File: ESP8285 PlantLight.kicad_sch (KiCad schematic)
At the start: 43 parts, among them J1 Screw_Terminal_01x01, J2 Screw_Terminal_01x01, Q1 P-Chan Mosfet, U1 ESP8285, U2 RT9193-33GB, Y1 26Mhz

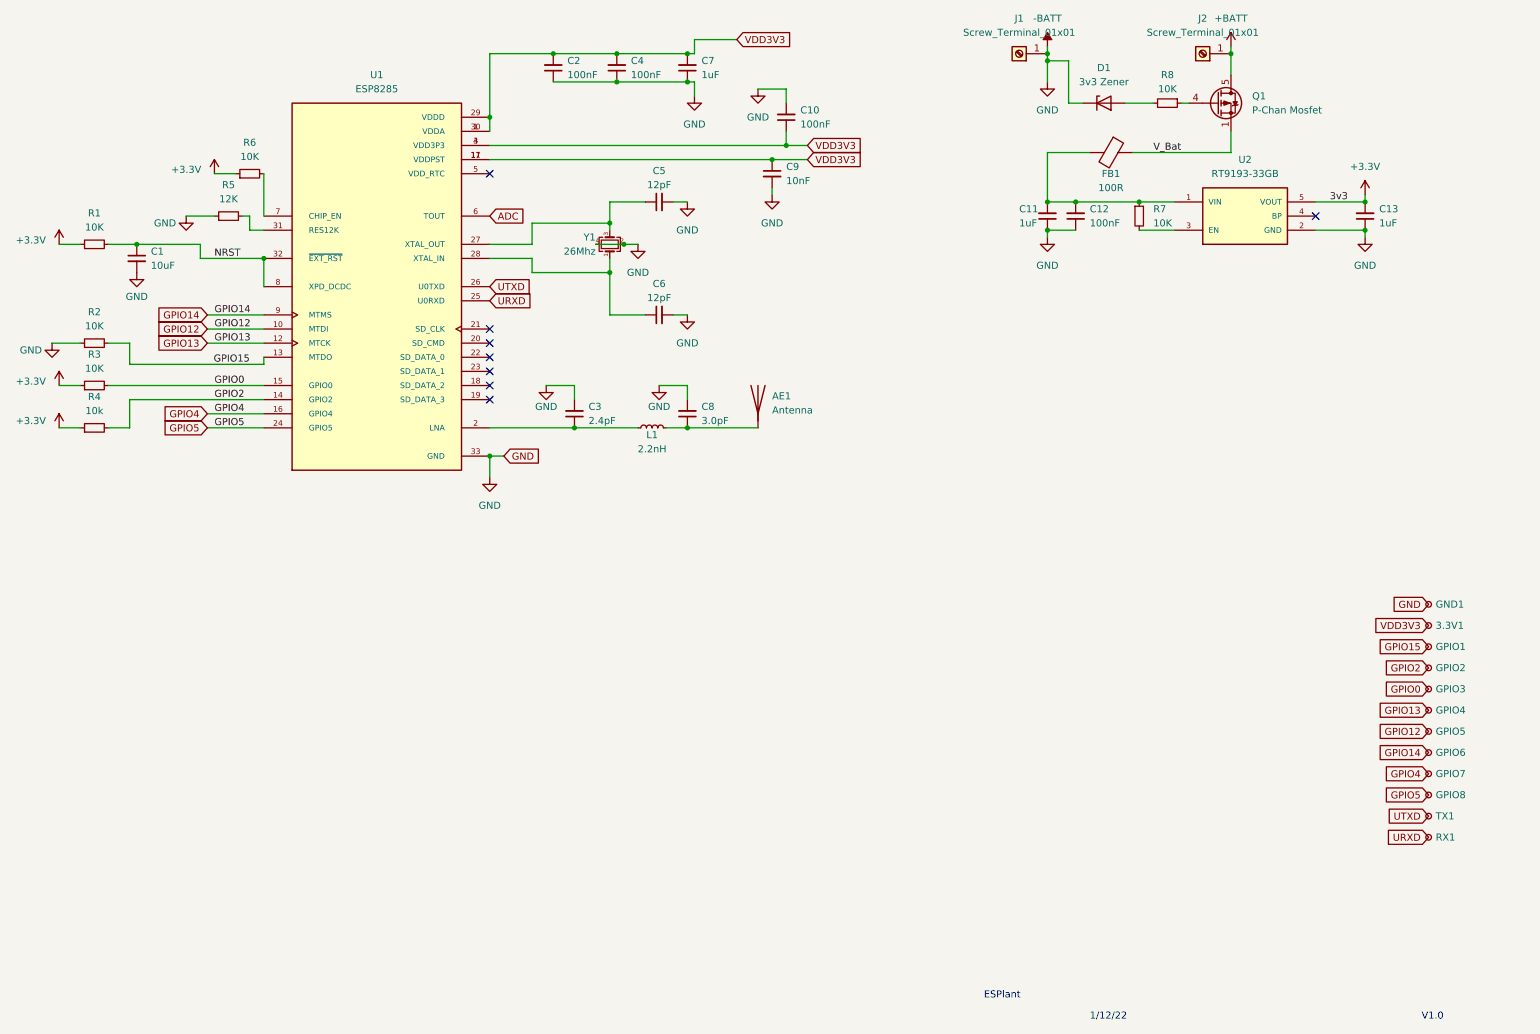
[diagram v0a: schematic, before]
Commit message: sat session
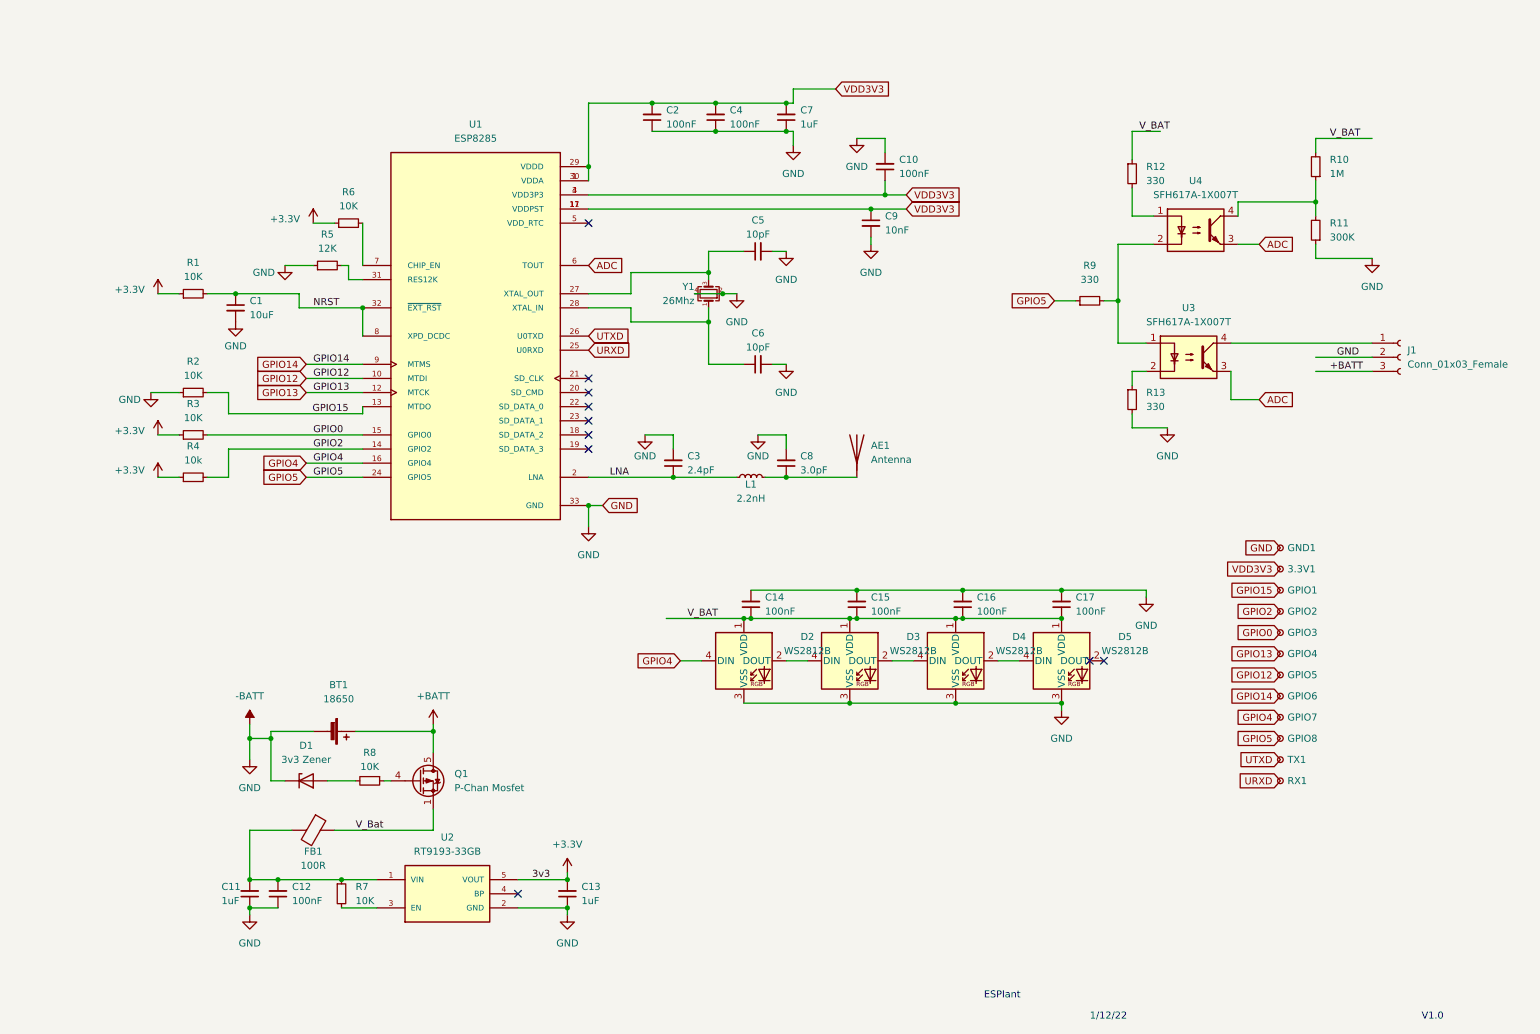
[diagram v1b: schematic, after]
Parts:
- removed J1, J2: Screw_Terminal_01x01, Library:Keystone_16mm_19mm_18650, symbol Connector:Screw_Terminal_01x01
- added BT1: 18650, Library:18650_footprint, symbol Device:Battery_Cell
- added C14, C15, C16, C17: 100nF, Capacitor_SMD:C_0402_1005Metric, symbol Device:C_Small
- added D2, D3, D4, D5: WS2812B, LED_SMD:LED_WS2812B_PLCC4_5.0x5.0mm_P3.2mm, symbol LED:WS2812B
- added J1: Conn_01x03_Female, Connector_PinHeader_2.54mm:PinHeader_1x03_P2.54mm_Vertical, symbol Connector:Conn_01x03_Female
- added R10: 1M, Capacitor_SMD:C_0402_1005Metric, symbol Device:R_Small
- added R11: 300K, symbol Device:R_Small
- added R12, R13, R9: 330, Capacitor_SMD:C_0402_1005Metric, symbol Device:R_Small
- added U3, U4: SFH617A-1X007T, Package_DIP:SMDIP-4_W9.53mm_Clearance8mm, symbol Isolator:SFH617A-1X007T
- C12: footprint (none) -> Capacitor_SMD:C_0402_1005Metric
- C2, C4: footprint Capacitor_SMD:C_0603_1608Metric -> Capacitor_SMD:C_0402_1005Metric
- C5, C6: value 12pF -> 10pF
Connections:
- net +BATT: now also BT1.1 (+), J1.3 (Pin_3)
- net -BATT: now also BT1.2 (-), C14.2, C15.2, C16.2, C17.2, D2.3 (VSS), D3.3 (VSS), D4.3 (VSS), D5.3 (VSS), J1.2 (Pin_2), R11.1, R13.2
- net ADC: now also U3.3, U4.3
- net GPIO4: now also D2.4 (DIN)
- net GPIO5: now also R9.1
- net LNA: now reaches C3.1, L1.1, U1.2 (LNA)
- new net: R12.2, U4.1
- new net: R9.2, U3.1, U4.2
- new net: R10.1, R11.2, U4.4
- new net: R13.1, U3.2
- new net: D3.2 (DOUT), D4.4 (DIN)
- new net: D2.2 (DOUT), D3.4 (DIN)
- new net: J1.1 (Pin_1), U3.4
- new net: D4.2 (DOUT), D5.4 (DIN)
- new net V_BAT: C14.1, C15.1, C16.1, C17.1, D2.1 (VDD), D3.1 (VDD), D4.1 (VDD), D5.1 (VDD), R10.2, R12.1
- no-connect marks 8 -> 10
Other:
- moved on the sheet: 3.3V1, AE1, C1, C10, C11, C12, C13, C2, C3, C4, C5, C6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
